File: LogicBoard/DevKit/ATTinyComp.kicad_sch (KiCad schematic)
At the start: 11 parts, among them J21 UARTDBG, U1 TPL0401B-10DCKR, U2 ATTINY1616-MNR

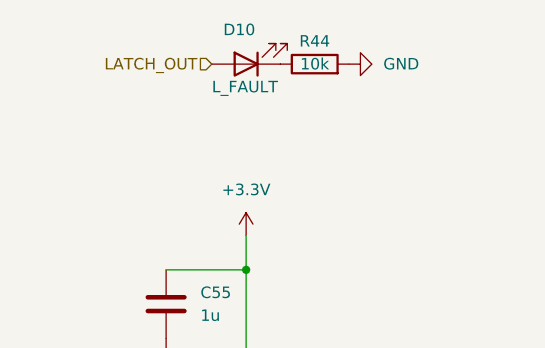
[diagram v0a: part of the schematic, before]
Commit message: v3.2.2 - TL494V2
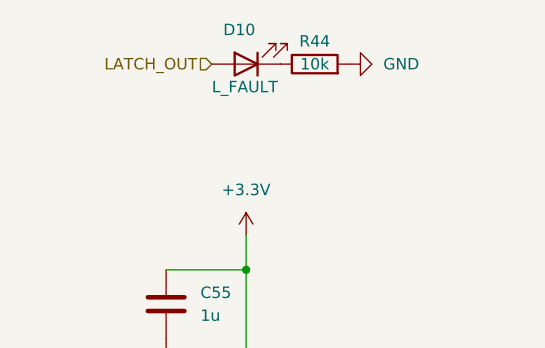
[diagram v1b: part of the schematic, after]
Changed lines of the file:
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@@
 			)
 		)
-		(property "Description" ""
+		(property "Description" "Power symbol creates a global label with name \"GND\" , ground"
 			(at 144.78 111.76 0)
 			(effects
@@
 			)
 		)
-		(property "Description" ""
+		(property "Description" "Power symbol creates a global label with name \"+3.3V\""
 			(at 71.12 83.82 0)
 			(effects
@@
 			)
 		)
-		(property "Description" ""
+		(property "Description" "Power symbol creates a global label with name \"GND\" , ground"
 			(at 92.71 104.14 0)
 			(effects
@@
 			)
 		)
-		(property "Description" ""
+		(property "Description" "Power symbol creates a global label with name \"+3.3V\""
 			(at 72.39 46.99 0)
 			(effects
@@
 			)
 		)
-		(property "Description" ""
+		(property "Description" "Power symbol creates a global label with name \"+3.3V\""
 			(at 144.78 49.53 0)
 			(effects
@@
 			)
 		)
-		(property "Description" ""
+		(property "Description" "Power symbol creates a global label with name \"GND\" , ground"
 			(at 135.89 60.96 0)
 			(effects
@@
 			)
 		)
-		(property "Description" ""
+		(property "Description" "Power symbol creates a global label with name \"+3.3V\""
 			(at 72.39 40.64 0)
 			(effects
@@
 			)
 		)
-		(property "Description" ""
+		(property "Description" "Power symbol creates a global label with name \"GND\" , ground"
 			(at 71.12 109.22 0)
 			(effects
@@
 		)
 		(property "Value" "GND"
-			(at 160.02 30.48 90)
+			(at 160.02 30.4799 90)
 			(effects
 				(font
@@
 			)
 		)
-		(property "Description" ""
+		(property "Description" "Power symbol creates a global label with name \"GND\" , ground"
 			(at 156.21 30.48 0)
 			(effects
